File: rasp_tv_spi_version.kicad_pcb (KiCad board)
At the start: 2 copper layers, 118.3 x 53.5 mm, 12 parts, among them J1 Raspberry_Pi_2_3, J6 PAM8302-input, J7 PAM8302-output, J8 SPEAKER, J9 5V_USB, SW1 SW_Push_DPDT, U1 TFT_320x240

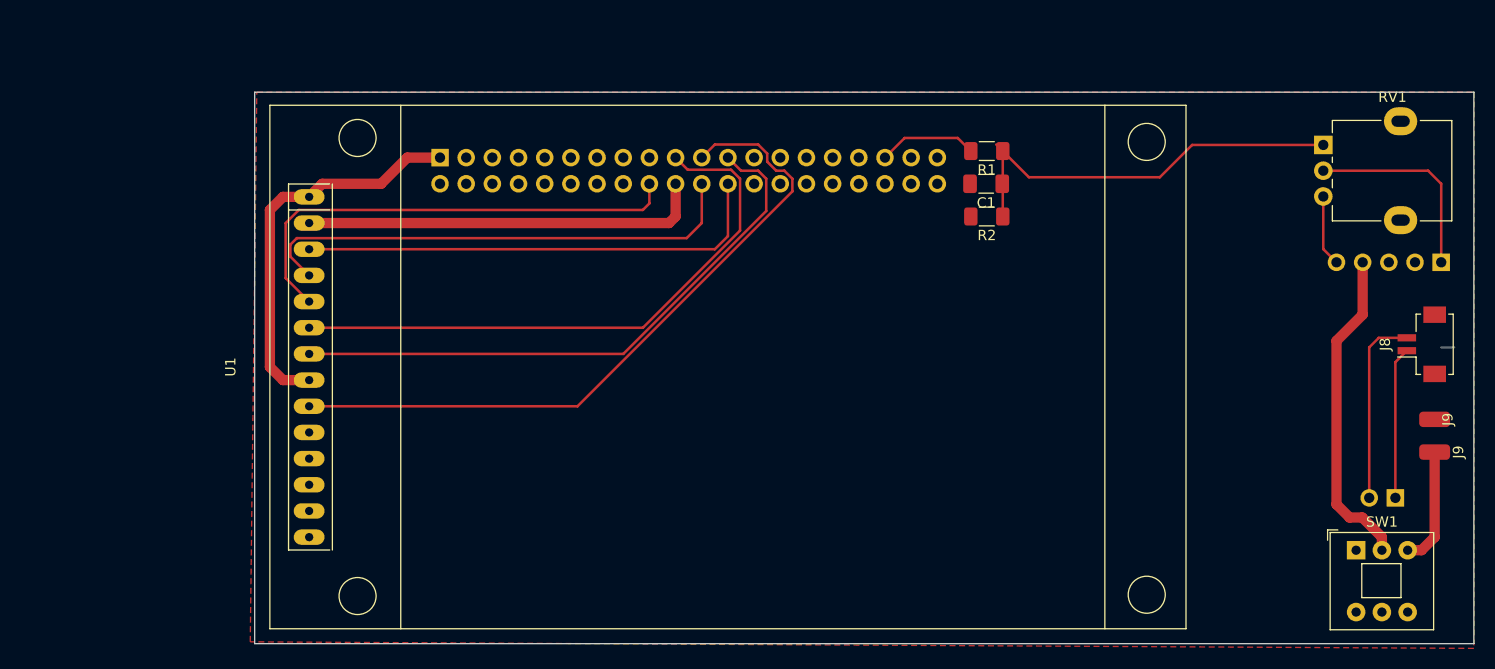
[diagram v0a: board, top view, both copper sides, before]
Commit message: make pcb routing
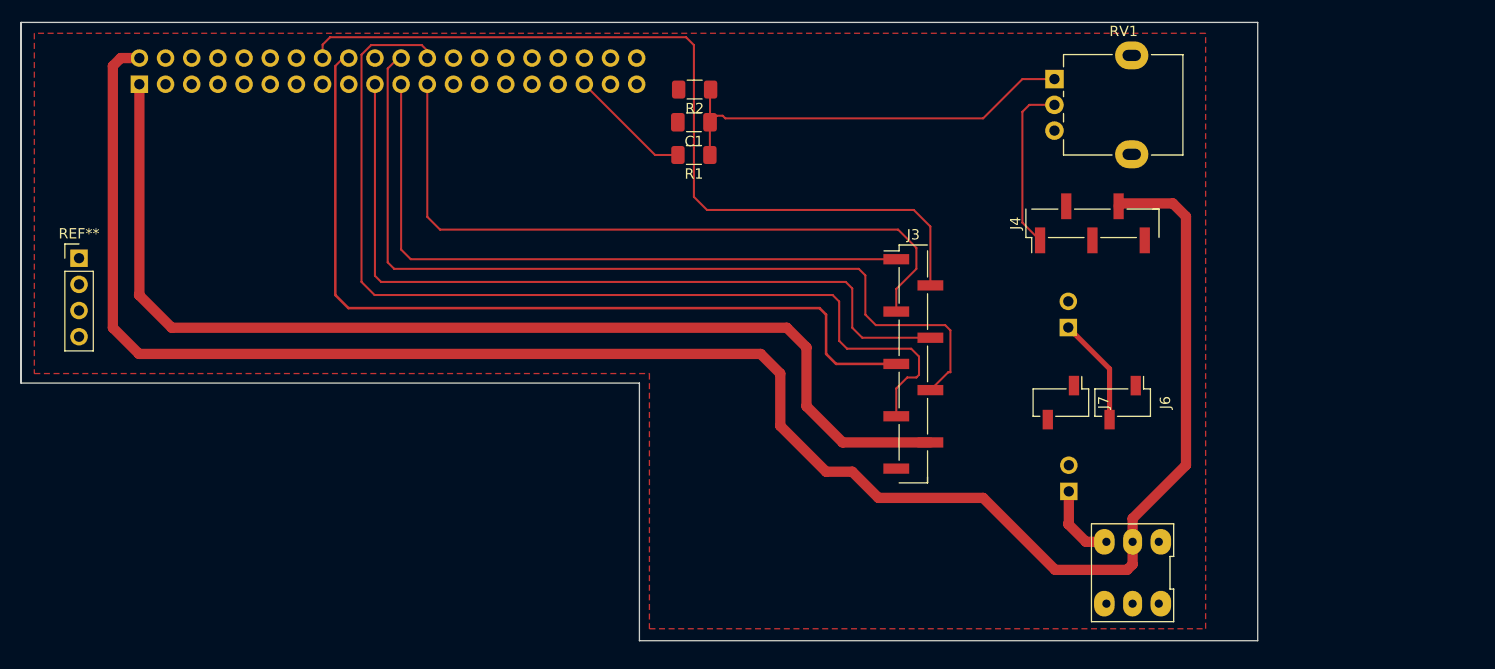
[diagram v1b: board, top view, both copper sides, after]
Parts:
- removed J9 (x2): 5V_USB, Connector_Wire:SolderWirePad_1x01_SMD_1.5x3mm
- removed U1: TFT_320x240, Display:TFT-320x240
- added J3: Conn_01x09, Connector_PinHeader_2.54mm:PinHeader_1x09_P2.54mm_Vertical_SMD_Pin1Left, F.Cu at (166.6, 91.1)
- added J4: AUODIO_IN, Connector_PinHeader_2.54mm:PinHeader_1x05_P2.54mm_Vertical_SMD_Pin1Left, F.Cu at (184.0, 77.5)
- added J5: SPEAKER, Connector_PinHeader_2.54mm:PinHeader_1x02_P2.54mm_Horizontal, B.Cu at (181.6, 87.6)
- added REF**: PinHeader_1x04_P2.54mm_Vertical, Connector_PinHeader_2.54mm:PinHeader_1x04_P2.54mm_Vertical, F.Cu at (85.6, 80.9)
- J1: footprint Connector_PinHeader_2.54mm:PinHeader_2x20_P2.54mm_Vertical -> Connector_PinSocket_2.54mm:PinSocket_2x20_P2.54mm_Vertical
- J6: value PAM8302-input -> AUDIO_OUT; footprint Connector_PinHeader_2.54mm:PinHeader_1x05_P2.54mm_Vertical -> Connector_PinSocket_2.54mm:PinSocket_1x02_P2.54mm_Vertical_SMD_Pin1Left; moved to F.Cu
- J7: value PAM8302-output -> AUDIO_OUT; footprint Connector_PinHeader_2.54mm:PinHeader_1x02_P2.54mm_Vertical -> Connector_PinSocket_2.54mm:PinSocket_1x02_P2.54mm_Vertical_SMD_Pin1Left; moved to F.Cu
- J8: value SPEAKER -> Conn_01x02_Pin; footprint Connector_Hirose:Hirose_DF13C_CL535-0402-2-51_1x02-1MP_P1.25mm_Vertical -> Connector_PinHeader_2.54mm:PinHeader_1x02_P2.54mm_Horizontal; moved to B.Cu
- SW1: footprint Button_Switch_THT:SW_Push_2P2T_Toggle_CK_PVA2OAH5xxxxxxV2 -> Button_Switch_THT:SW_DPDT_XLX
- moved J8 37.1 mm to (181.7, 103.5), turned to 0 degrees
- moved J6 33.8 mm to (186.9, 94.9), turned to -90 degrees
- moved J7 33.8 mm to (180.9, 94.9), turned to -90 degrees
- moved R2 30.9 mm to (145.4, 64.5)
- moved J1 30.0 mm to (91.5, 64.0)
- moved C1 29.0 mm to (145.3, 67.7)
- moved R1 28.4 mm to (145.3, 70.9)
- moved RV1 26.9 mm to (180.3, 63.5)
- moved SW1 21.8 mm to (187.9, 111.4), turned to 180 degrees
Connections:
- J1 pad 16: unconnected-(J1-GPIO23-Pad16) -> BACKLIGHT_23_GPIO
- J6 pad 1: Net-(J6-Pin_1) -> unconnected-(J6-Pin_1-Pad1)
- J6 pad 2: GND -> Net-(J5-Pin_1)
- J7 pad 1: Net-(J7-Pin_1) -> Net-(J5-Pin_2)
- J7 pad 2: Net-(J7-Pin_2) -> unconnected-(J7-Pin_2-Pad2)
- J8 pad 1: Net-(J7-Pin_1) -> Net-(J8-Pin_1)
- J8 pad 2: Net-(J7-Pin_2) -> Net-(J8-Pin_2)
- RV1 pad : GND -> (no net)
- RV1 pad 2: Net-(J6-Pin_1) -> AUDIO_IN
- SW1 pad 3: Net-(J9-Pin_2) -> Net-(J8-Pin_1)
- SW1 pad 4: unconnected-(SW1-A-Pad4) -> Net-(J8-Pin_2)
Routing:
- net +5V: track 31.5 -> 183.3 mm
- net BACKLIGHT_23_GPIO: track 0.00 -> 82.5 mm
- net +3.3V: track 38.2 -> 106.5 mm
- net CS_8_GPIO: track 46.2 -> 96.3 mm
- net GND: track 45.9 -> 0.00 mm
- net RESET_25_GPIO: track 48.3 -> 86.8 mm
- net DC_24_GPIO: track 46.6 -> 83.3 mm
- net Net-(J6-Pin_1): track 19.6 -> 0.00 mm
- net MOSI_0_10_GPIO: track 57.9 -> 77.3 mm
- net Net-(J7-Pin_2): track 18.6 -> 0.00 mm
- net AUDIO_IN: track 0.00 -> 16.6 mm
- net Net-(J7-Pin_1): track 14.7 -> 0.00 mm
- net Net-(J9-Pin_2): track 11.4 -> 0.00 mm
- net SCK_0_11_GPIO: track 57.8 -> 68.6 mm
- net Net-(J5-Pin_1): track 0.00 -> 10.6 mm
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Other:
- board size 118.3 x 53.5 mm -> 120 x 60 mm
